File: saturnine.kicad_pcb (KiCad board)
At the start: 2 copper layers, 99.1 x 79.9 mm, 27 parts, among them SW10 SW_Push, SW11 SW_Push, SW12 SW_Push, SW14 SW_Push, SW15 SW_Push, SW16 SW_Push, SW17 SW_Push, SW18 SW_Push, SW2 SW_Push, SW20 SW_Push, SW21 SW_Push, SW3 SW_Push, SW4 SW_Push, SW5 SW_Push, SW6 SW_Push, SW8 SW_Push, SW9 SW_Push, U1 ProMicro-kbd

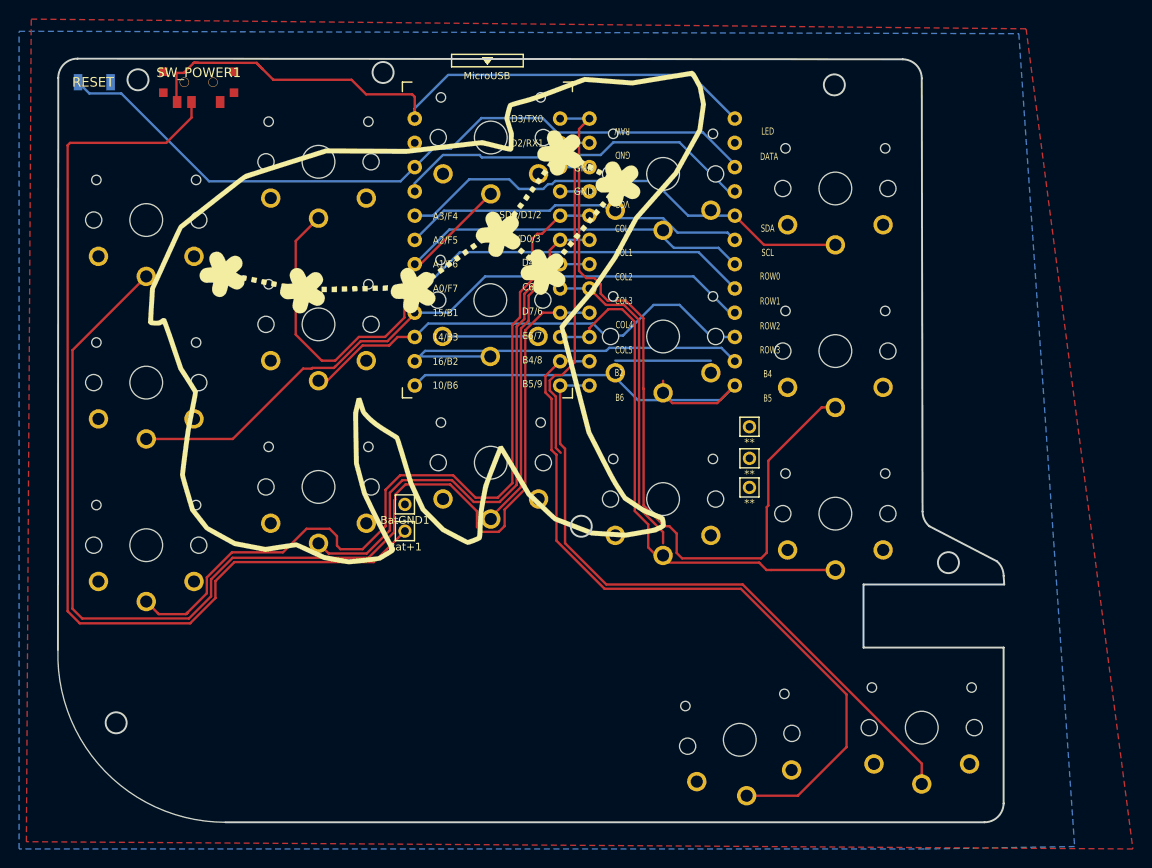
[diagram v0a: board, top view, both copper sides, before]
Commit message: commit correct files
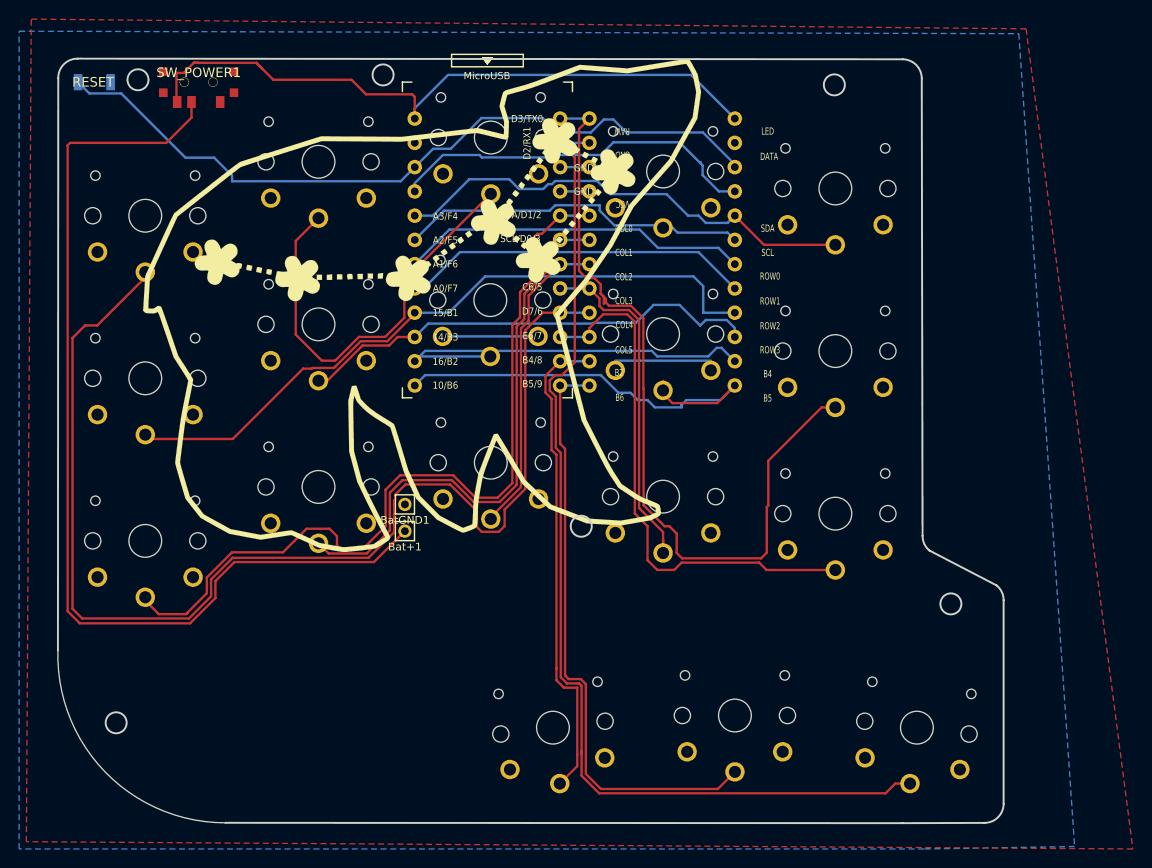
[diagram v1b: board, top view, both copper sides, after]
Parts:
- removed ** (x3): Val**, kbd:1pin_conn
- added SW22: SW_Push, Kailh:SW_PG1350_rev_DPB, F.Cu at (110.5, 88.1)
- moved SW21 19.6 mm to (91.4, 86.9)
- moved SW20 19.6 mm to (72.4, 88.1)
- moved G*** 1.37 mm to (58.7, 43.9)
- moved SW14 0.46 mm to (29.7, 68.6)
- moved SW2 0.46 mm to (29.7, 34.6)
- moved SW8 0.46 mm to (29.7, 51.6)
- moved SW11 0.25 mm to (83.9, 46.9)
- moved SW17 0.25 mm to (83.9, 64.0)
- moved SW5 0.25 mm to (83.9, 29.9)
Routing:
- net Switch18: track 38.1 -> 109.4 mm
- net Switch16: track 78.1 -> 51.0 mm
- net Switch17: track 69.9 -> 62.6 mm
- net Switch14: track 34.1 -> 36.0 mm
- net Switch6: track 70.3 -> 71.9 mm
- net reset: track 78.1 -> 79.6 mm
- net Switch10: track 84.1 -> 85.5 mm
- net Switch15: track 54.9 -> 55.9 mm
- net Switch9: track 46.4 -> 47.2 mm
- net Switch1: track 124.9 -> 125.6 mm
- net vcc: track 38.5 -> 39.2 mm
- net Switch5: track 49.1 -> 49.8 mm
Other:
- board size 99.1 x 79.9 mm -> 99 x 80 mm
- net class Default removed
- board text added: "Jupiter or Thor is perfect. We need Atlas for our long-distance stuff."
- board text added: "The Titan will be even better."
